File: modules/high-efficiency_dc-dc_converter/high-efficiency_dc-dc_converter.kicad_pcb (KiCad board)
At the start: 2 copper layers, 29.5 x 22.5 mm, 13 parts

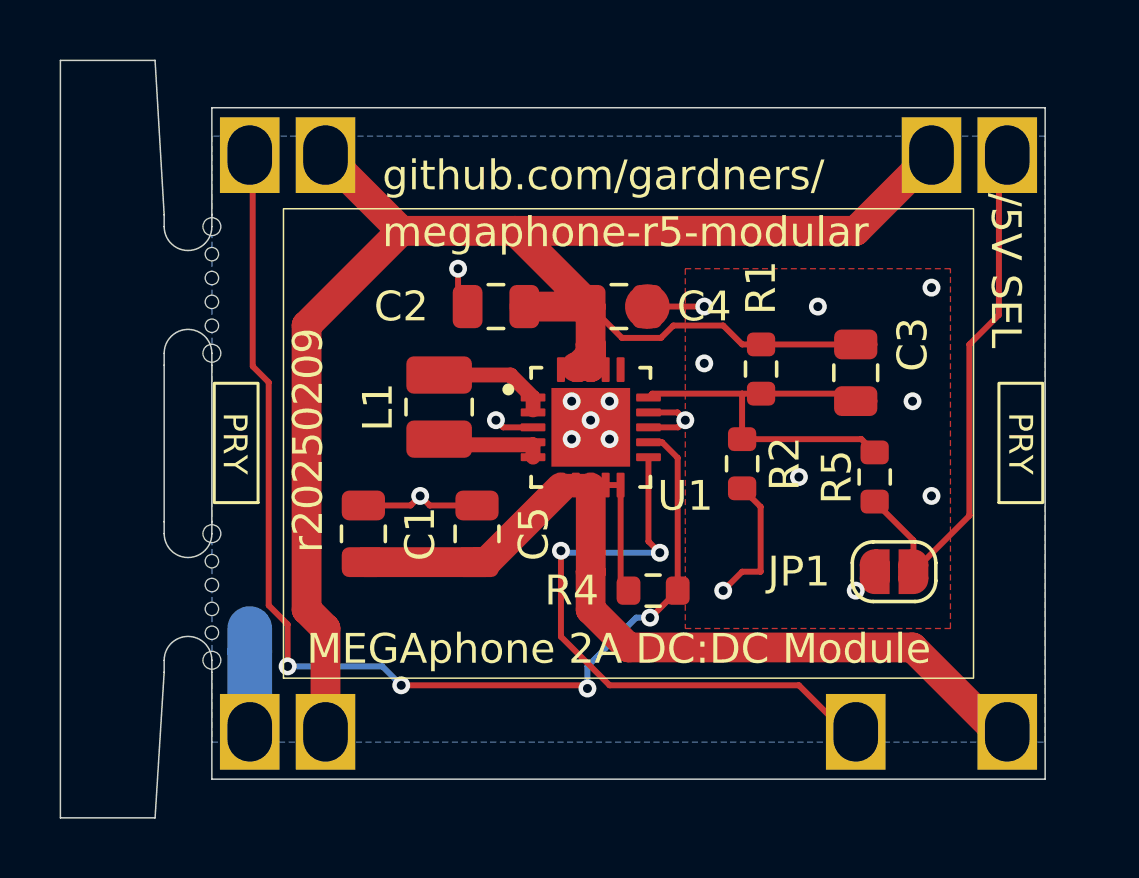
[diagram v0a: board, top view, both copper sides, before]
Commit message: Updating high-efficiency_dc-dc_converter
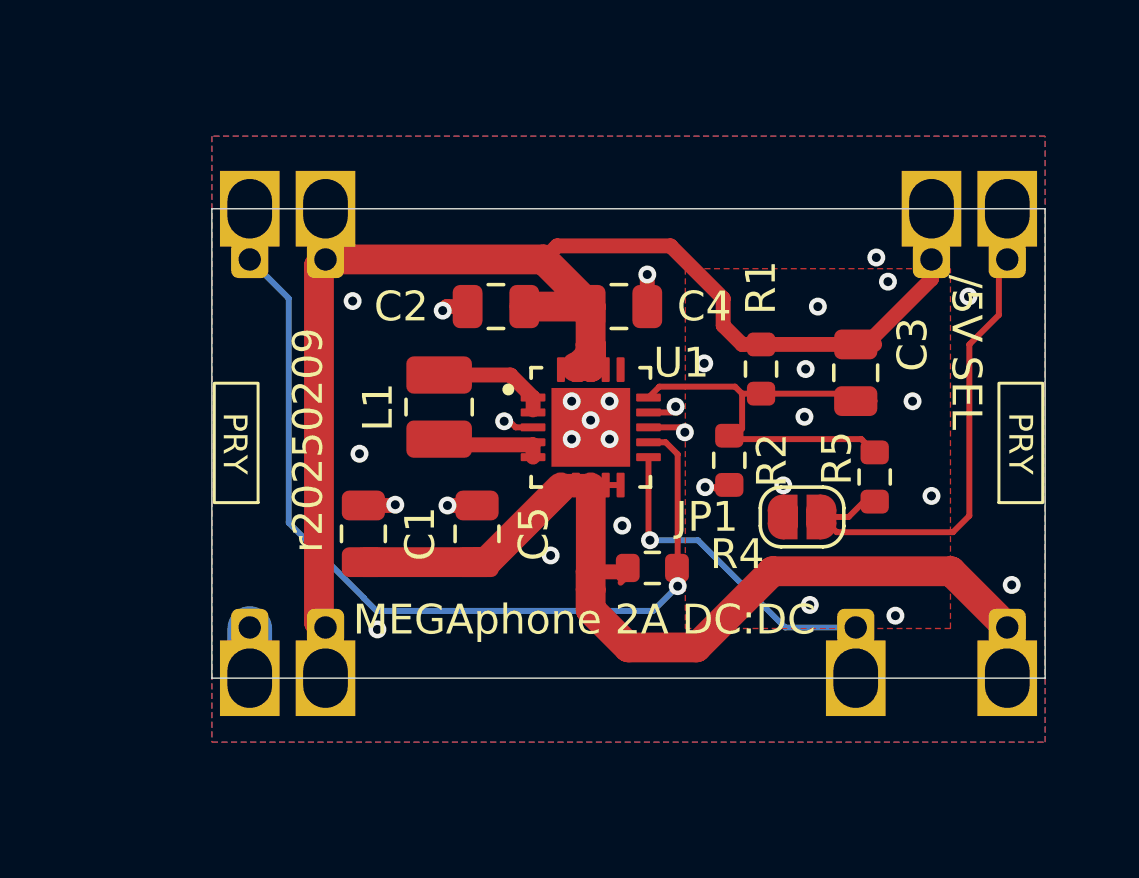
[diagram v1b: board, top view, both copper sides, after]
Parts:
- M1: footprint MegaCastle:MegaCastle2x11-Module-I15.7x23.1-MA0780C-PANEL-NIBBLE -> MegaCastle:MegaCastle2x11-Module-I15.7x23.1-MA0780C-SPAREPAD
- U1: value ~ -> ISl91127IR; footprint QFN20:QFN50P400X400X90-21N -> MegaCastle:QFN50P400X400X90-21N
- moved JP1 3.59 mm to (69.3, 43.2)
- moved R4 0.76 mm to (64.3, 45.0)
- moved R2 0.45 mm to (66.9, 41.4)
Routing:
- net VCC_OUT: track 60.4 -> 44.7 mm
- net GND: track 19.8 -> 9.24 mm, vias 18 -> 31
- net EN: track 20.9 -> 11.0 mm, vias 2 -> 1
- net MODE: track 39.3 -> 29.6 mm, vias 4 -> 1
- net /5V_SEL: track 19.0 -> 16.7 mm
- net VBAT: track 32.9 -> 31.7 mm
- net Net-(U1-FB): track 13.9 -> 14.7 mm
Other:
- board size 29.5 x 22.5 mm -> 27.9 x 15.7 mm
- board text added: "MEGAphone 2A DC:DC"
